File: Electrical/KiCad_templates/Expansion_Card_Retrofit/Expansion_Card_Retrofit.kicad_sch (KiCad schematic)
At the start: 14 parts, among them J1 Conn 10P, P1 USB_C_Plug_USB2.0, SW1 SW_DIP_x03, U1 AP2112K-3.3, X1 ECS-2520MVLC-120-CM-TR

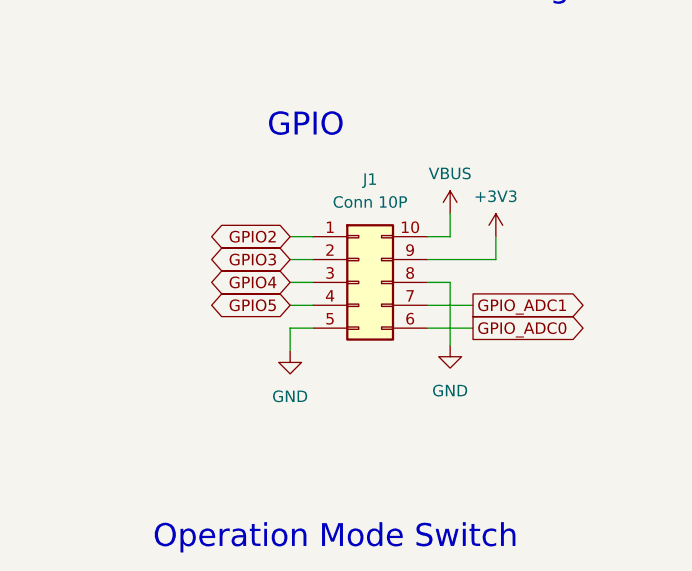
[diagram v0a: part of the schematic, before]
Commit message: Current state before flash footprint update
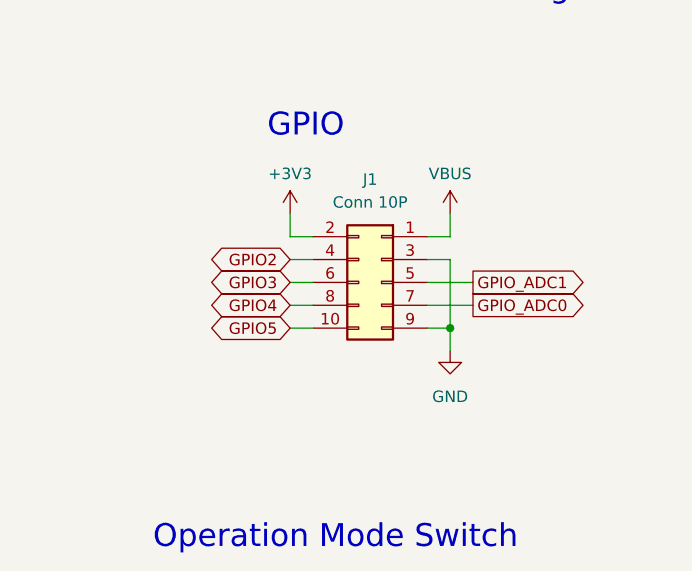
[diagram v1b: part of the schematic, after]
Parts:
- J1: footprint Connector_PinSocket_2.54mm:PinSocket_2x05_P2.54mm_Horizontal -> SnapEDA:AMPHENOL_89883-405LF; symbol Connector_Generic:Conn_02x05_Counter_Clockwise -> Connector_Generic:Conn_02x05_Odd_Even
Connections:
- net +3V3: now also J1.2 (Pin_2); no longer J1.9 (Pin_9)
- net GND: now also J1.3 (Pin_3), J1.9 (Pin_9); no longer J1.5 (Pin_5), J1.8 (Pin_8)
- net GPIO2: now also J1.4 (Pin_4); no longer J1.1 (Pin_1)
- net GPIO3: now also J1.6 (Pin_6); no longer J1.2 (Pin_2)
- net GPIO4: now also J1.8 (Pin_8); no longer J1.3 (Pin_3)
- net GPIO5: now also J1.10 (Pin_10); no longer J1.4 (Pin_4)
- net GPIO_ADC0: now also J1.7 (Pin_7); no longer J1.6 (Pin_6)
- net GPIO_ADC1: now also J1.5 (Pin_5); no longer J1.7 (Pin_7)
- net VBUS: now also J1.1 (Pin_1); no longer J1.10 (Pin_10)

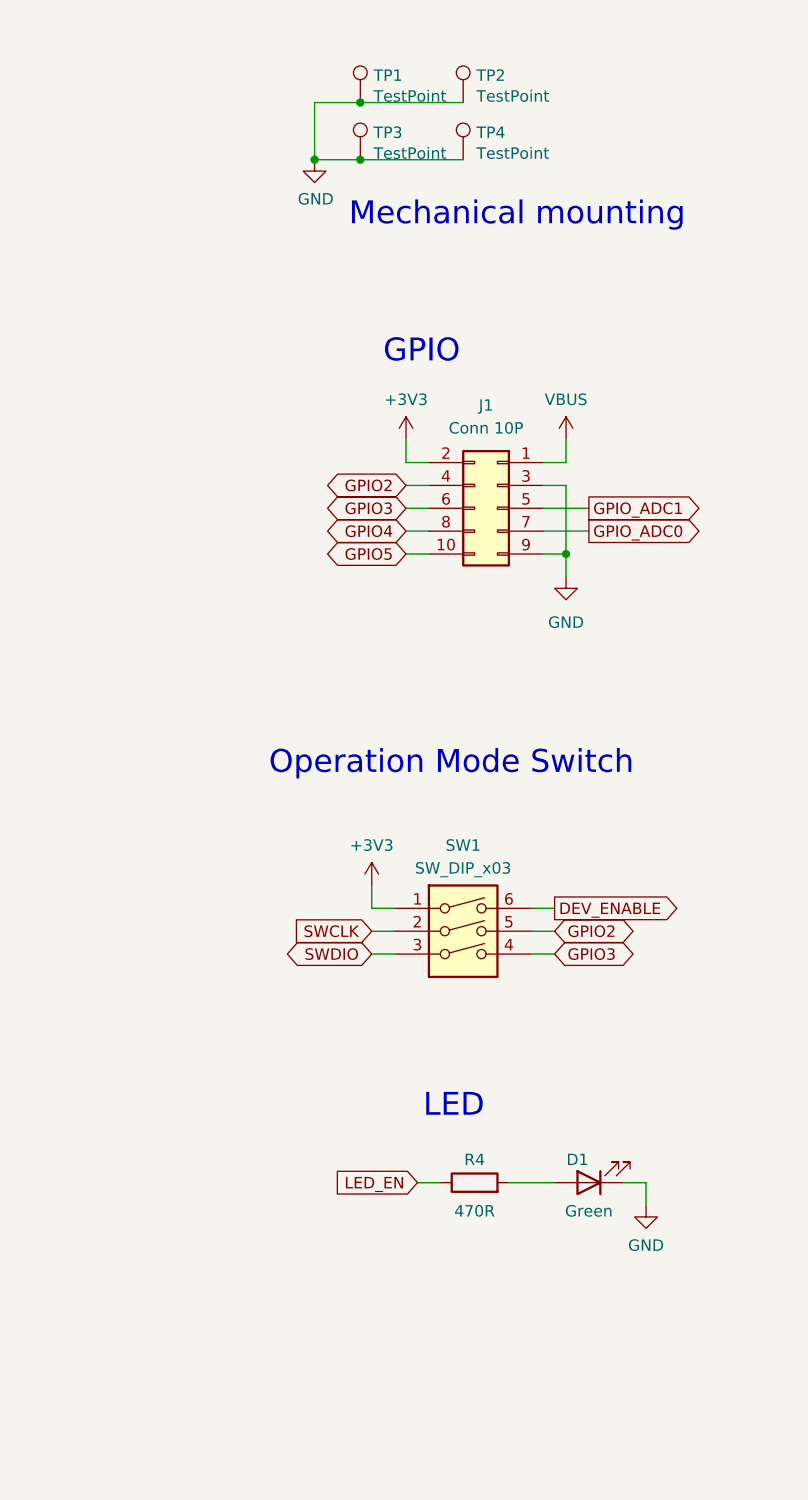
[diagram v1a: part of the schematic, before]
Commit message: First complete version
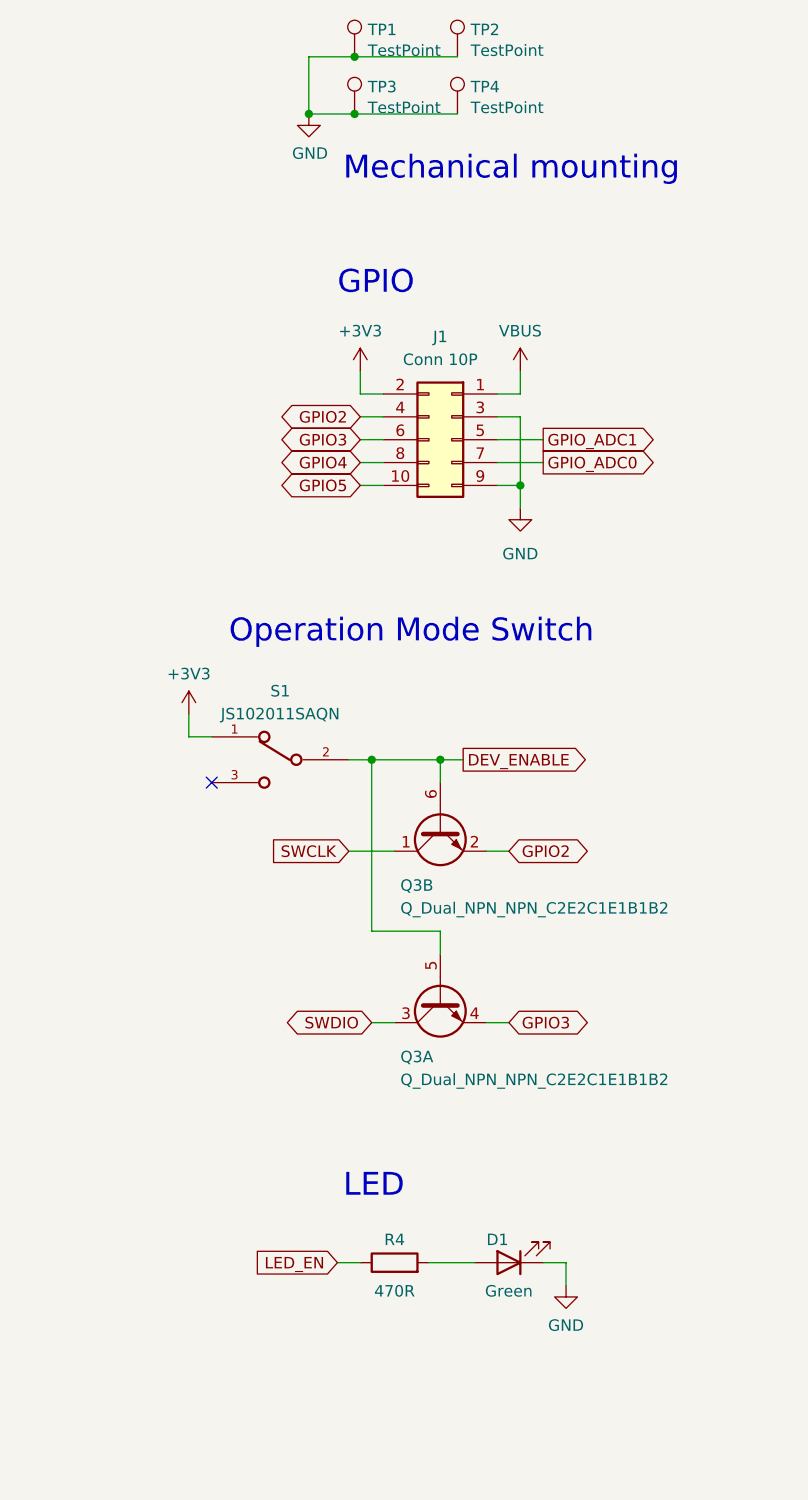
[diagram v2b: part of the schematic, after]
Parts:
- removed SW1: SW_DIP_x03, symbol Switch:SW_DIP_x03
- added Q3: Q_Dual_NPN_NPN_C2E2C1E1B1B2, digikey-footprints:SOT-363, symbol Device:Q_Dual_NPN_NPN_C2E2C1E1B1B2
- added S1: JS102011SAQN, SnapEDA:SW_JS102011SAQN, symbol SnapEDA:JS102011SAQN
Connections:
- net +3V3: now also S1.1
- net DEV_ENABLE: now also Q3.5 (B1), Q3.6 (B2), S1.2
- net GPIO2: now also Q3.2 (E2)
- net GPIO3: now also Q3.4 (E1)
- net SWCLK: now also Q3.1 (C2)
- net SWDIO: now also Q3.3 (C1)
- no-connect marks 2 -> 3
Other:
- moved on the sheet: D1, J1, R4, TP1, TP2, TP3, TP4
